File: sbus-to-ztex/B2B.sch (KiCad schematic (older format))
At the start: 6 parts, among them J3 Conn_02x07_Odd_Even

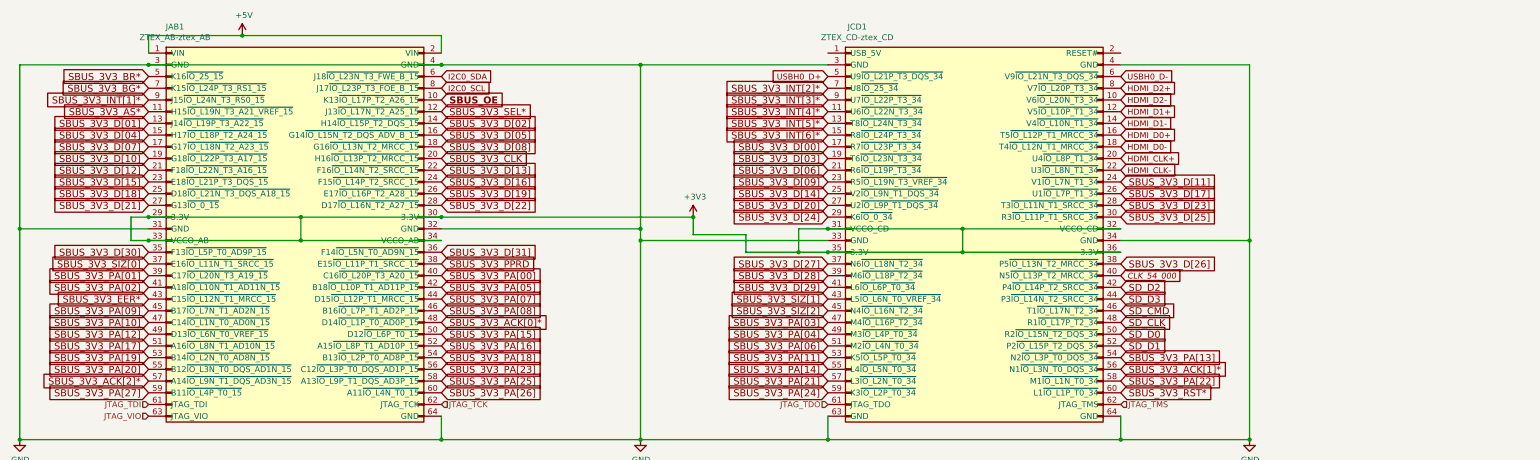
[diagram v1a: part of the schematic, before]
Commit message: more V1.3
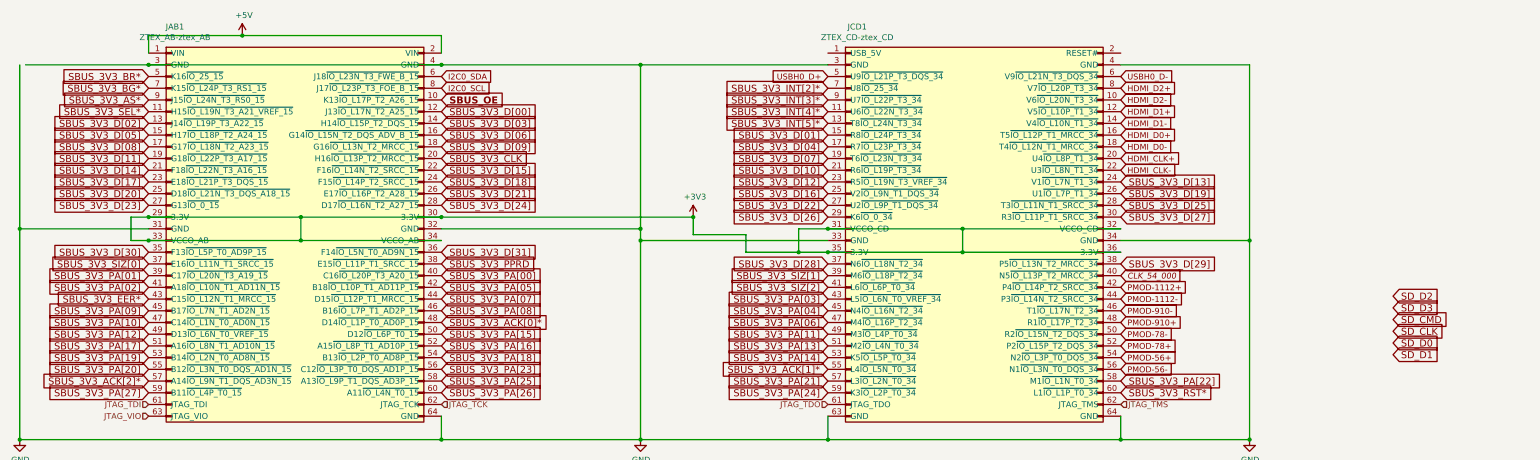
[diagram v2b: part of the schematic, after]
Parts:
- JAB1, JCD1: DNP (none) -> DNP
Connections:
- net labels added: PMOD-1112+, PMOD-1112-, PMOD-56+, PMOD-56-, PMOD-78+, PMOD-78-, PMOD-910+, PMOD-910-
- net labels removed: SBUS_3V3_INT[1]*, SBUS_3V3_INT[6]*
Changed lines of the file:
@@
 F 4 "10-89-7642" H 1800 2650 50  0001 C CNN "MPN"
 F 5 "https://www2.mouser.com/ProductDetail/Molex/10-89-7642?qs=%2Fha2pyFadugCxzQFZUdvioDcljDVidgd4vXrOFuSRYM%3D" H 1800 2650 50  0001 C CNN "URL"
+F 6 "DNP" H 1800 2650 50  0001 C CNN "DNP"
 	1    1800 2650
 	1    0    0    -1
@@
 Text Notes 9950 6500 0    50   ~ 0
 Clock capable inputs (MRCC and SRCC, MRCC are multi-domain)\nFor 2.13:\nB9 G16~IO_L13N_T2_MRCC_15 G16\nB10 H16~IO_L13P_T2_MRCC_15 H16\nB11 F16~IO_L14N_T2_SRCC_15 F16\nB12 F15~IO_L14P_T2_SRCC_15 F15\nA19 E16~IO_L11N_T1_SRCC_15 E16\nB19 E15~IO_L11P_T1_SRCC_15 E15\nA22 C15~IO_L12N_T1_MRCC_15 C15\nB22 D15~IO_L12P_T1_MRCC_15 D15\nD8 T5~IO_L12P_T1_MRCC_34 T5\nD9 T4~IO_L12N_T1_MRCC_34 T4\nD14 T3~IO_L11N_T1_SRCC_34 T3\nD15 R3~IO_L11P_T1_SRCC_34 R3\nD19 P5~IO_L13N_T2_MRCC_34 P5\nD20 N5~IO_L13P_T2_MRCC_34 N5\nD21 P4~IO_L14P_T2_SRCC_34 P4\nD22 P3~IO_L14N_T2_SRCC_34 P3\n\nUnfortunately various 2.1x modules have different clock assignment. B22 hsould be a P-side MRCC for 2.14 (perhaps 2.18), but is a n-side SRCC on 2.16 so not usable there.
-Text GLabel 4100 2050 2    60   Input ~ 0
-SBUS_3V3_CLK
 Wire Wire Line
 	1450 2550 1450 2750
@@
 Wire Wire Line
 	7150 2850 6700 2850
-Text GLabel 7400 1950 0    60   Input ~ 0
-SBUS_3V3_D[00]
-Text GLabel 1600 1750 0    60   Input ~ 0
-SBUS_3V3_D[01]
-Text GLabel 4100 1750 2    60   Input ~ 0
-SBUS_3V3_D[02]
-Text GLabel 7400 2050 0    60   Input ~ 0
-SBUS_3V3_D[03]
-Text GLabel 1600 1850 0    60   Input ~ 0
-SBUS_3V3_D[04]
-Text GLabel 4100 1850 2    60   Input ~ 0
-SBUS_3V3_D[05]
-Text GLabel 7400 2150 0    60   Input ~ 0
-SBUS_3V3_D[06]
-Text GLabel 1600 1950 0    60   Input ~ 0
-SBUS_3V3_D[07]
+Text GLabel 1600 2150 0    60   Input ~ 0
+SBUS_3V3_D[14]
+Text GLabel 4100 1950 2    60   Input ~ 0
+SBUS_3V3_D[09]
+Text GLabel 1600 2050 0    60   Input ~ 0
+SBUS_3V3_D[11]
 Text GLabel 1600 2250 0    60   Input ~ 0
-SBUS_3V3_D[15]
-Text GLabel 7400 2350 0    60   Input ~ 0
-SBUS_3V3_D[14]
-Text GLabel 4100 2150 2    60   Input ~ 0
-SBUS_3V3_D[13]
-Text GLabel 1600 2150 0    60   Input ~ 0
-SBUS_3V3_D[12]
-Text GLabel 7400 2250 0    60   Input ~ 0
-SBUS_3V3_D[09]
-Text GLabel 4100 1950 2    60   Input ~ 0
-SBUS_3V3_D[08]
-Text GLabel 9900 2250 2    60   Input ~ 0
-SBUS_3V3_D[11]
-Text GLabel 1600 2050 0    60   Input ~ 0
-SBUS_3V3_D[10]
-Text GLabel 4100 2250 2    60   Input ~ 0
-SBUS_3V3_D[16]
-Text GLabel 9900 2350 2    60   Input ~ 0
 SBUS_3V3_D[17]
 Text GLabel 1600 2350 0    60   Input ~ 0
-SBUS_3V3_D[18]
-Text GLabel 4100 2350 2    60   Input ~ 0
-SBUS_3V3_D[19]
-Text GLabel 7400 2450 0    60   Input ~ 0
 SBUS_3V3_D[20]
 Text GLabel 1600 2450 0    60   Input ~ 0
-SBUS_3V3_D[21]
-Text GLabel 4100 2450 2    60   Input ~ 0
-SBUS_3V3_D[22]
-Text GLabel 9900 2450 2    60   Input ~ 0
 SBUS_3V3_D[23]
 Text GLabel 4100 2850 2    60   Input ~ 0
@@
 Text GLabel 1600 2850 0    60   Input ~ 0
 SBUS_3V3_D[30]
-Text GLabel 7400 3150 0    60   Input ~ 0
+Text GLabel 9900 2950 2    60   Input ~ 0
 SBUS_3V3_D[29]
-Text GLabel 7400 3050 0    60   Input ~ 0
-SBUS_3V3_D[28]
-Text GLabel 7400 2950 0    60   Input ~ 0
+Text GLabel 9900 2550 2    60   Input ~ 0
 SBUS_3V3_D[27]
-Text GLabel 9900 2950 2    60   Input ~ 0
+Text GLabel 7400 2550 0    60   Input ~ 0
 SBUS_3V3_D[26]
-Text GLabel 9900 2550 2    60   Input ~ 0
+Text GLabel 9900 2450 2    60   Input ~ 0
 SBUS_3V3_D[25]
-Text GLabel 7400 2550 0    60   Input ~ 0
+Text GLabel 4100 2450 2    60   Input ~ 0
 SBUS_3V3_D[24]
-Text GLabel 7400 1850 0    60   Input ~ 0
-SBUS_3V3_INT[6]*
 Text GLabel 7400 1750 0    60   Input ~ 0
 SBUS_3V3_INT[5]*
@@
 Text GLabel 7400 1450 0    60   Input ~ 0
 SBUS_3V3_INT[2]*
-Text GLabel 1600 1550 0    60   Input ~ 0
-SBUS_3V3_INT[1]*
 Text GLabel 4100 3050 2    60   Input ~ 0
 SBUS_3V3_PA[00]
@@
 Text GLabel 1600 3150 0    60   Input ~ 0
 SBUS_3V3_PA[02]
+Text GLabel 7400 3250 0    60   Input ~ 0
+SBUS_3V3_PA[03]
+Text GLabel 7400 3350 0    60   Input ~ 0
+SBUS_3V3_PA[04]
 Text GLabel 7400 3450 0    60   Input ~ 0
-SBUS_3V3_PA[03]
-Text GLabel 7400 3550 0    60   Input ~ 0
-SBUS_3V3_PA[04]
-Text GLabel 7400 3650 0    60   Input ~ 0
 SBUS_3V3_PA[06]
 Text GLabel 4100 3250 2    60   Input ~ 0
@@
 Text GLabel 4100 3550 2    60   Input ~ 0
 SBUS_3V3_PA[15]
-Text GLabel 7400 3850 0    60   Input ~ 0
+Text GLabel 7400 3750 0    60   Input ~ 0
 SBUS_3V3_PA[14]
-Text GLabel 9900 3750 2    60   Input ~ 0
+Text GLabel 7400 3650 0    60   Input ~ 0
 SBUS_3V3_PA[13]
 Text GLabel 1600 3550 0    60   Input ~ 0
 SBUS_3V3_PA[12]
-Text GLabel 7400 3750 0    60   Input ~ 0
+Text GLabel 7400 3550 0    60   Input ~ 0
 SBUS_3V3_PA[11]
 Text GLabel 1600 3450 0    60   Input ~ 0
@@
 Text GLabel 1600 2950 0    60   Input ~ 0
 SBUS_3V3_SIZ[0]
-Text GLabel 7400 3250 0    60   Input ~ 0
+Text GLabel 7400 3050 0    60   Input ~ 0
 SBUS_3V3_SIZ[1]
-Text GLabel 7400 3350 0    60   Input ~ 0
+Text GLabel 7400 3150 0    60   Input ~ 0
 SBUS_3V3_SIZ[2]
 Text GLabel 1600 1350 0    60   Input ~ 0
 SBUS_3V3_BR*
-Text GLabel 4100 1650 2    60   Input ~ 0
-SBUS_3V3_SEL*
 Text GLabel 1600 1450 0    60   Input ~ 0
 SBUS_3V3_BG*
-Text GLabel 1600 1650 0    60   Input ~ 0
-SBUS_3V3_AS*
 Text GLabel 1600 3950 0    60   Input ~ 0
 SBUS_3V3_ACK[2]*
-Text GLabel 9900 3850 2    60   Input ~ 0
+Text GLabel 7400 3850 0    60   Input ~ 0
 SBUS_3V3_ACK[1]*
 Text GLabel 4100 3450 2    60   Input ~ 0
@@
 Text GLabel 1600 3250 0    60   Input ~ 0
 SBUS_3V3_EER*
-Text GLabel 9900 3150 2    60   Input ~ 0
+Text GLabel 12225 3225 2    60   Input ~ 0
 SD_D2
-Text GLabel 9900 3250 2    60   Input ~ 0
+Text GLabel 12225 3325 2    60   Input ~ 0
 SD_D3
-Text GLabel 9900 3350 2    60   Input ~ 0
+Text GLabel 12225 3425 2    60   Input ~ 0
 SD_CMD
-Text GLabel 9900 3450 2    60   Input ~ 0
+Text GLabel 12225 3525 2    60   Input ~ 0
 SD_CLK
-Text GLabel 9900 3550 2    60   Input ~ 0
+Text GLabel 12225 3625 2    60   Input ~ 0
 SD_D0
-Text GLabel 9900 3650 2    60   Input ~ 0
+Text GLabel 12225 3725 2    60   Input ~ 0
 SD_D1
 $Comp
@@
 F 4 "10-89-7642" H 7600 2650 50  0001 C CNN "MPN"
 F 5 "https://www2.mouser.com/ProductDetail/Molex/10-89-7642?qs=%2Fha2pyFadugCxzQFZUdvioDcljDVidgd4vXrOFuSRYM%3D" H 7600 2650 50  0001 C CNN "URL"
+F 6 "DNP" H 7600 2650 50  0001 C CNN "DNP"
 	1    7600 2650
 	1    0    0    -1
@@
 Wire Wire Line
 	500  2650 1600 2650
-Wire Wire Line
-	1600 1250 4100 1250
-Wire Wire Line
-	1600 1250 500  1250
 Wire Wire Line
 	500  1250 500  2650
@@
 Text GLabel 9900 3050 2    50   Input Italic 0
 CLK_54_000
+Wire Wire Line
+	1600 1250 550  1250
+Wire Wire Line
+	1600 1250 4100 1250
+Text GLabel 1600 1550 0    60   Input ~ 0
+SBUS_3V3_AS*
+Text GLabel 4100 2350 2    60   Input ~ 0
+SBUS_3V3_D[21]
+Text GLabel 4100 2250 2    60   Input ~ 0
+SBUS_3V3_D[18]
+Text GLabel 7400 2150 0    60   Input ~ 0
+SBUS_3V3_D[10]
+Text GLabel 7400 2250 0    60   Input ~ 0
+SBUS_3V3_D[12]
+Text GLabel 4100 2150 2    60   Input ~ 0
+SBUS_3V3_D[15]
+Text GLabel 7400 2050 0    60   Input ~ 0
+SBUS_3V3_D[07]
+Text GLabel 7400 1950 0    60   Input ~ 0
+SBUS_3V3_D[04]
+Text GLabel 7400 1850 0    60   Input ~ 0
+SBUS_3V3_D[01]
+Text GLabel 7400 2950 0    60   Input ~ 0
+SBUS_3V3_D[28]
+Text GLabel 1600 1650 0    60   Input ~ 0
+SBUS_3V3_SEL*
+Text GLabel 7400 2450 0    60   Input ~ 0
+SBUS_3V3_D[22]
+Text GLabel 9900 2350 2    60   Input ~ 0
+SBUS_3V3_D[19]
+Text GLabel 7400 2350 0    60   Input ~ 0
+SBUS_3V3_D[16]
+Text GLabel 9900 2250 2    60   Input ~ 0
+SBUS_3V3_D[13]
+Text GLabel 1600 1850 0    60   Input ~ 0
+SBUS_3V3_D[05]
+Text GLabel 1600 1750 0    60   Input ~ 0
+SBUS_3V3_D[02]
+Text GLabel 4100 2050 2    60   Input ~ 0
+SBUS_3V3_CLK
+Text GLabel 1600 1950 0    60   Input ~ 0
+SBUS_3V3_D[08]
+Text GLabel 4100 1850 2    60   Input ~ 0
+SBUS_3V3_D[06]
+Text GLabel 4100 1750 2    60   Input ~ 0
+SBUS_3V3_D[03]
+Text GLabel 4100 1650 2    60   Input ~ 0
+SBUS_3V3_D[00]
+Text GLabel 9900 3850 2    50   Input ~ 0
+PMOD-56-
+Text GLabel 9900 3550 2    50   Input ~ 0
+PMOD-78-
+Text GLabel 9900 3350 2    50   Input ~ 0
+PMOD-910-
+Text GLabel 9900 3250 2    50   Input ~ 0
+PMOD-1112-
+Text GLabel 9900 3150 2    50   Input ~ 0
+PMOD-1112+
+Text GLabel 9900 3750 2    50   Input ~ 0
+PMOD-56+
+Text GLabel 9900 3650 2    50   Input ~ 0
+PMOD-78+
+Text GLabel 9900 3450 2    50   Input ~ 0
+PMOD-910+
 $EndSCHEMATC
